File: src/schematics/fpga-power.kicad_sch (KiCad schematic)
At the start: 47 parts, among them U6 LFE5U-85F-*BG756*

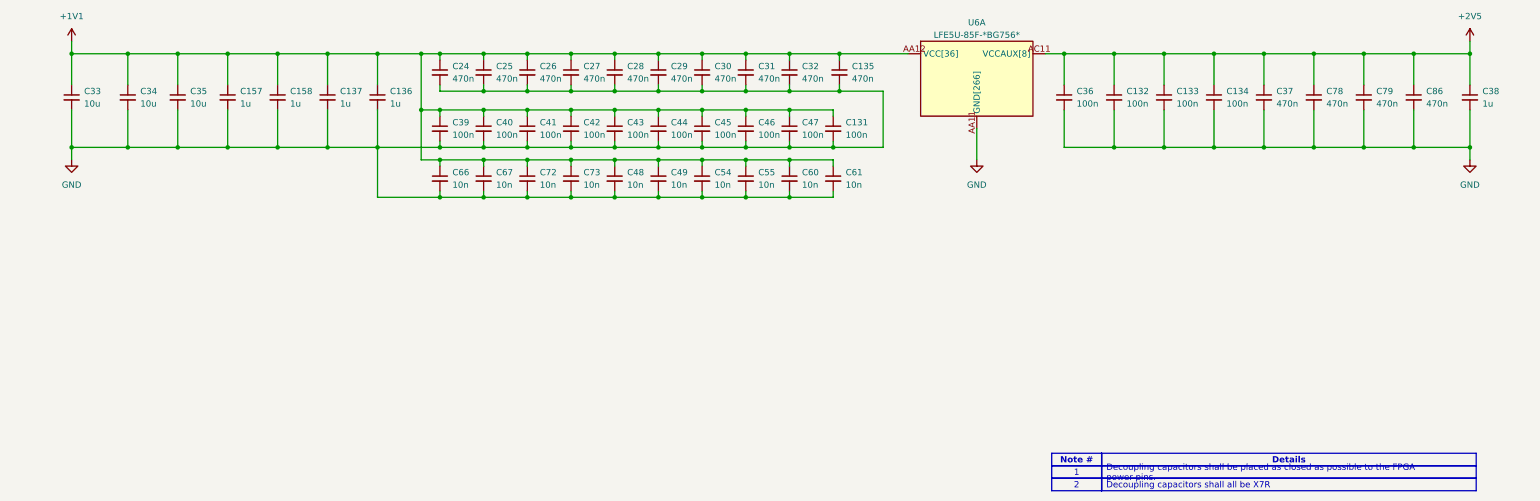
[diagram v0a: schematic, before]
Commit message: Add bom components
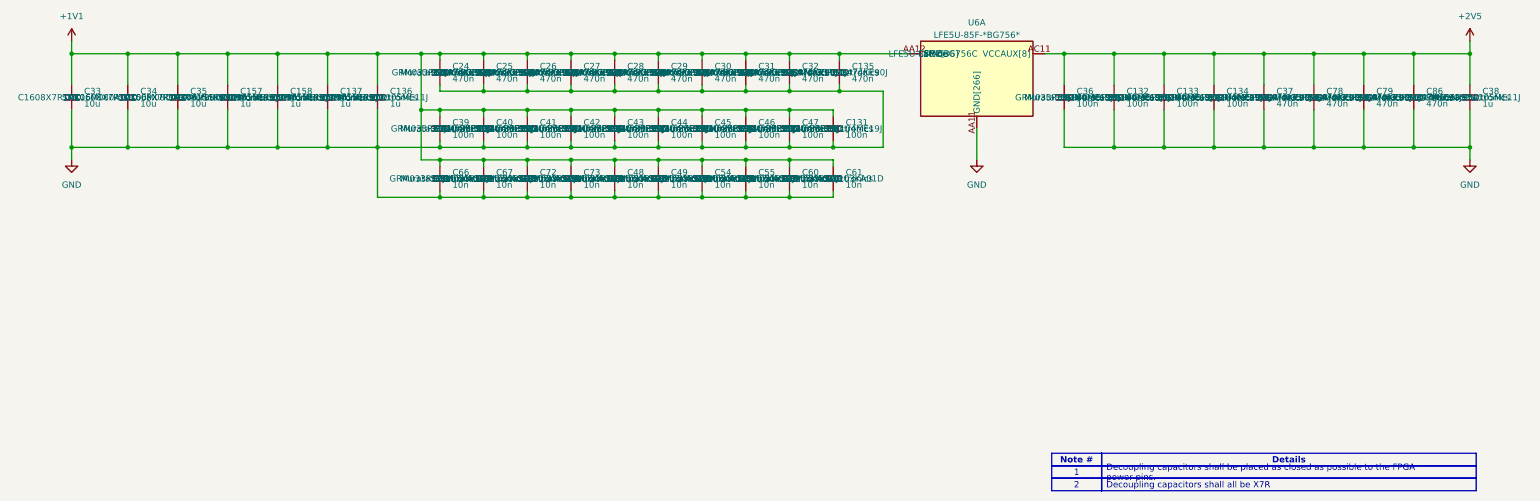
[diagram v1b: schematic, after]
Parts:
- C131, C132, C133, C134, C36, C39, C40, C41, C42, C43, C44, C45, C46, C47: MPN (none) -> GRM033R60J104ME19J; Manufacturer (none) -> Murata Electronics; Mouting Technology (none) -> SMD
- C135, C24, C25, C26, C27, C28, C29, C30, C31, C32, C37, C78, C79, C86: MPN (none) -> GRM033R60J474KE90J; Manufacturer (none) -> Murata Electronics; Mouting Technology (none) -> SMD
- C136, C137, C157, C158, C38: MPN (none) -> GRM155R6YA105ME11J; Manufacturer (none) -> Murata Electronics; Mouting Technology (none) -> SMD
- C33, C34, C35: MPN (none) -> C1608X7R1A106M080AT; Manufacturer (none) -> TDK; Mouting Technology (none) -> SMD
- C48, C49, C54, C55, C60, C61, C66, C67, C72, C73: MPN (none) -> GRM033R60J103KA01D; Manufacturer (none) -> Murata Electronics; Mouting Technology (none) -> SMD
- U6: MPN (none) -> LFE5U-85F-6BG756C; Manufacturer (none) -> Lattice; Mouting Technology (none) -> SMD
